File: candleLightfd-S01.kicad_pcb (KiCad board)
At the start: 2 copper layers, 37.7 x 20 mm, 45 parts, among them P1 CONN_01X02, P2 CONN_01X02, T101 Tab, T102 Tab, T103 Tab, T104 Tab, U1 STM32G0B1CBT, U2 MCP1754ST-3302E/MB, U3 TJA1051T3, U4 TJA1051T3, X1 629722000214_pasteInHole, X3 TC2030-NL, Y1 830055299

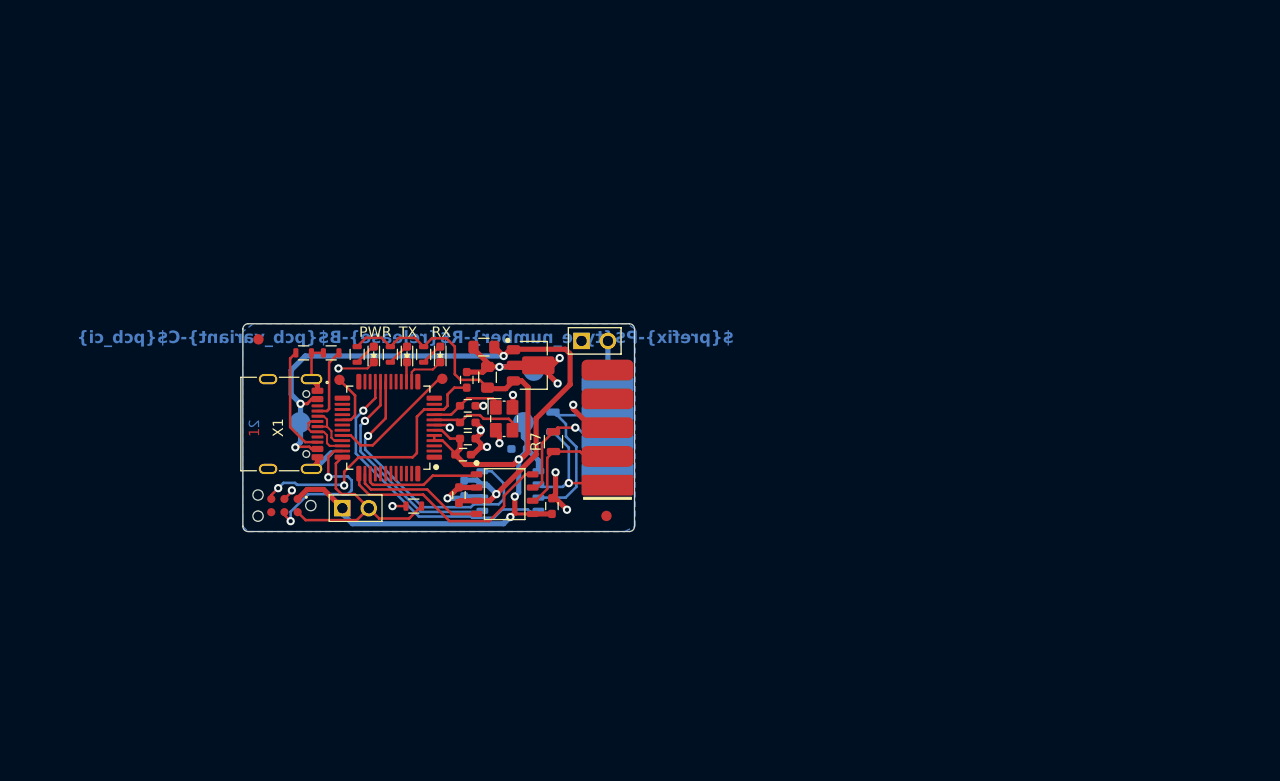
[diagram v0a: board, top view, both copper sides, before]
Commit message: clean up
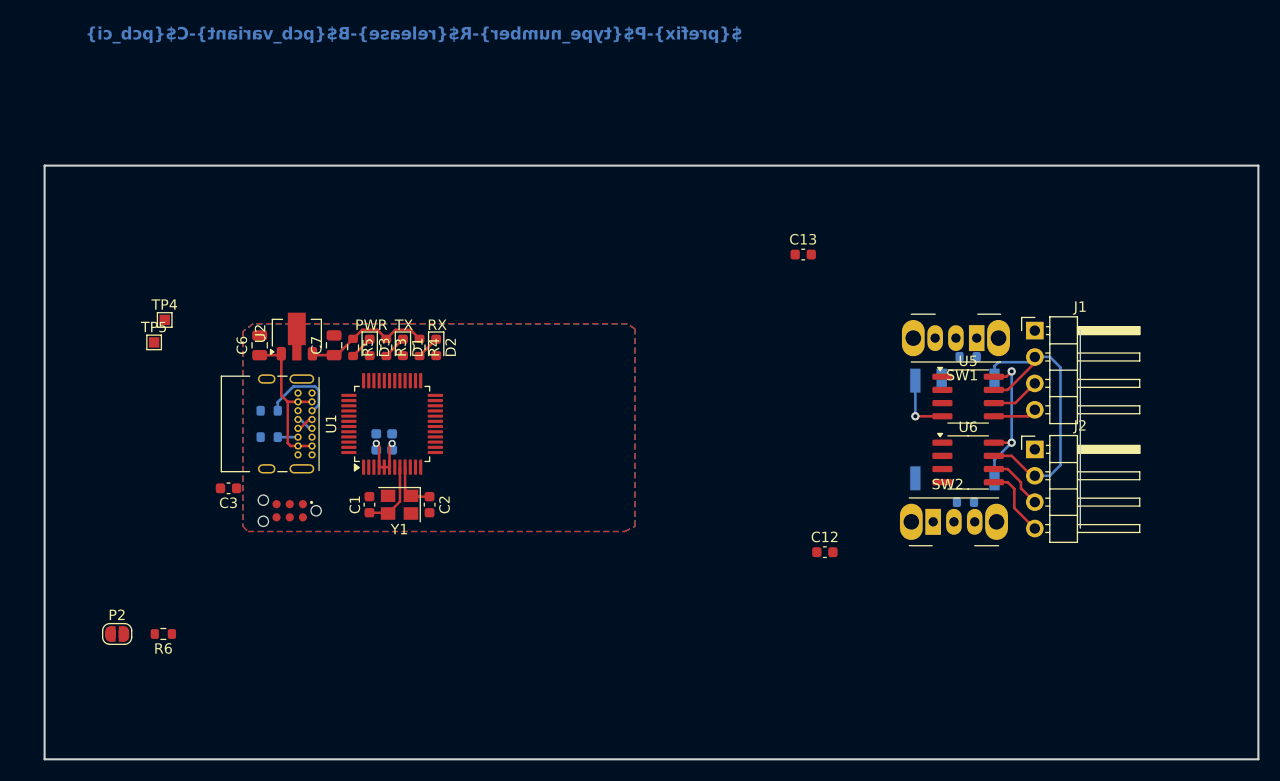
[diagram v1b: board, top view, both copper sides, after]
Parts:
- removed C10, C11, C8, C9: 100n_0603_X7R_10%_50V_-40C..125C_Chip-Capacitor, Capacitors_SMD:C_0603
- removed NB2: LAYERSTACK_TB, mechanical:LAYERSTACK_TB
- removed NB3, NB4: Passermarke_1mm_1.8mmx1.8mm, mechanical:Passermarke_1mm_1.8mmx1.8mm
- removed P1: CONN_01X02, Connector_generic:Header_1x2_Pitch2.54mm
- removed R1, R2: 5k1_0603_100mW_1%_E24_Chip-Resistor, Resistors_SMD:R_0603
- removed T101, T102, T103, T104: Tab, kikit:Tab
- removed TP1, TP2, TP3: TP2.0mm, Connector_generic:TP2.0mm
- removed U3, U4: TJA1051T3, tssop:SOIC-8_3.90mmx4.90mm_Pitch1.27mm
- removed X1: 629722000214_pasteInHole, Socket_GCT:USB4105_pasteInHole
- removed X2: ~, d-sub:D-SUB-9_side
- added C12: 100n_0603_X7R_10%_50V_-40C..125C_Chip-Capacitor, Capacitor_SMD:C_0603_1608Metric, F.Cu at (157.0, 142.0)
- added C13: 100n_0603_X7R_10%_50V_-40C..125C_Chip-Capacitor, Capacitor_SMD:C_0603_1608Metric, F.Cu at (154.9, 113.3)
- added J1: CAN1, Connector_PinHeader_2.54mm:PinHeader_1x04_P2.54mm_Horizontal, F.Cu at (177.2, 120.7)
- added J2: CAN2, Connector_PinHeader_2.54mm:PinHeader_1x04_P2.54mm_Horizontal, F.Cu at (177.2, 132.1)
- added J3: USB_C_Receptacle_USB2.0_16P, Connector_USB:USB_C_Receptacle_GCT_USB4085, F.Cu at (107.7, 126.7)
- added R10: 5k1_0603_100mW_1%_E24_Chip-Resistor, Resistor_SMD:R_0603_1608Metric, B.Cu at (103.5, 128.4)
- added R9: 5k1_0603_100mW_1%_E24_Chip-Resistor, Resistor_SMD:R_0603_1608Metric, B.Cu at (103.5, 130.9)
- added SW1: Term1, Button_Switch_THT:SW_Slide_SPDT_Angled_CK_OS102011MA1Q, F.Cu at (171.6, 121.4)
- added SW2: Term2, Button_Switch_THT:SW_Slide_SPDT_Angled_CK_OS102011MA1Q, F.Cu at (167.4, 139.1)
- added U5: ISO1044BD, Package_SO:SOIC-8_3.9x4.9mm_P1.27mm, F.Cu at (170.8, 127.0)
- added U6: ISO1044BD, Package_SO:SOIC-8_3.9x4.9mm_P1.27mm, F.Cu at (170.8, 133.3)
- added U7: NXE1S0505MC, Converter_DCDC:Converter_DCDC_Murata_NXExSxxxxMC_SMD, B.Cu at (170.8, 130.2)
- C1, C2, C3: footprint Capacitors_SMD:C_0603 -> Capacitor_SMD:C_0603_1608Metric
- C4, C5: footprint Capacitors_SMD:C_0603 -> Capacitor_SMD:C_0603_1608Metric; moved to B.Cu
- C6, C7: footprint Capacitors_SMD:C_0805 -> Capacitor_SMD:C_0805_2012Metric
- D1, D2, D3: footprint LEDs_Kingbright:LED_Kingbright_0603 -> LED_SMD:LED_0603_1608Metric
- P2: footprint Connector_generic:Header_1x2_Pitch2.54mm -> Jumper:SolderJumper-2_P1.3mm_Open_RoundedPad1.0x1.5mm
- R3, R4, R5, R6: footprint Resistors_SMD:R_0603 -> Resistor_SMD:R_0603_1608Metric
- R7: value 120R_0805_125mW_1%_E24_Chip-Resistor -> 120; footprint Resistors_SMD:R_0805 -> Resistor_SMD:R_0603_1608Metric; moved to B.Cu
- R8: value 120R_0805_125mW_1%_E24_Chip-Resistor -> 120; footprint Resistors_SMD:R_0805 -> Resistor_SMD:R_0603_1608Metric
- TP4, TP5: footprint Connector_generic:TP1.0mm -> TestPoint:TestPoint_Pad_1.0x1.0mm
- U1: footprint QFP:LQFP-48_7mmx7mm_Pitch0.5mm -> Package_QFP:LQFP-48_7x7mm_P0.5mm
- U2: footprint TO_SMD:SOT-89 -> Package_TO_SOT_SMD:SOT-89-3
- Y1: value 830055299 -> 830108313809; footprint crystal:Crystal_4Pin_SMD_3.2mmx2.5mm -> Crystal:Crystal_SMD_3225-4Pin_3.2x2.5mm
- moved NB1 79.4 mm to (45.1, 94.6)
- moved R7 40.7 mm to (170.8, 123.2), turned to 180 degrees
- moved R8 40.5 mm to (170.6, 137.2), turned to 180 degrees
- moved TP4 27.3 mm to (93.5, 119.6)
- moved P2 27.1 mm to (88.9, 149.9)
- moved R6 27.1 mm to (93.3, 149.9)
- moved C3 25.2 mm to (99.6, 135.8), turned to 180 degrees
- moved U2 23.0 mm to (106.2, 120.9), turned to 90 degrees
- moved C6 21.6 mm to (102.6, 122.1), turned to 90 degrees
- moved TP5 18.2 mm to (92.5, 121.8)
- moved C7 15.1 mm to (109.8, 122.1)
- moved Y1 13.0 mm to (116.1, 137.4), turned to 180 degrees
- moved C1 12.3 mm to (113.2, 137.4), turned to -90 degrees
- moved C2 10.2 mm to (119.0, 137.4), turned to 90 degrees
- moved C4 8.45 mm to (113.8, 131.4), turned to 90 degrees
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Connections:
- R7 pad 2: /CAN1_L -> Net-(SW1-B)
- R8 pad 2: /CAN2_L -> Net-(SW2-B)
- U1 pad 19: /CAN Transiver/CAN2_RX -> /CAN Transceiver/CAN2_RX
- U1 pad 20: /CAN Transiver/CAN2_TX -> /CAN Transceiver/CAN2_TX
- U1 pad 21: /CAN Transiver/CAN2_S -> unconnected-(U1B-PB2-Pad21)
- U1 pad 37: /CAN Transiver/CAN1_S -> unconnected-(U1A-PA15-Pad37)
- U1 pad 38: /CAN Transiver/CAN1_RX -> /CAN Transceiver/CAN1_RX
- U1 pad 39: /CAN Transiver/CAN1_TX -> /CAN Transceiver/CAN1_TX
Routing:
- net +3V3: track 83.2 -> 19.5 mm, vias 3 -> 2
- net +5V: track 65.2 -> 15.8 mm, vias 4 -> 0
- net GND: track 54.9 -> 6.09 mm, vias 16 -> 1
- net GNDD: track 0.00 -> 31.1 mm
- net /CAN Transiver/CAN2_S: track 28.3 -> 0.00 mm, vias 1 -> 0
- net /CAN Transiver/CAN2_RX: track 27.4 -> 0.00 mm, vias 1 -> 0
- net /MCU/NRST: track 27.2 -> 0.00 mm, vias 2 -> 0
- net /CAN Transiver/CAN1_S: track 21.7 -> 0.00 mm
- net /CAN Transiver/CAN2_TX: track 21.7 -> 0.00 mm, vias 1 -> 0
- net /MCU/SWCLK: track 20.9 -> 0.00 mm
- net /MCU/SWDIO: track 15.7 -> 0.00 mm, vias 2 -> 0
- net +5VD: track 0.00 -> 14.6 mm, vias 0 -> 2
- net /CAN Transiver/CAN1_RX: track 12.9 -> 0.00 mm
- net /MCU/RX: track 12.7 -> 0.00 mm
- net /CAN2_H: track 17.7 -> 5.60 mm
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- added copper zone on F.Cu, net GND
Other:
- board size 37.7 x 20 mm -> 116.8 x 57.2 mm
- board text removed: "+3V3"
- board text removed: "0"
- board text removed: "0 mm"
- board text removed: "0.01 mm"
- board text removed: "0.02"
- board text removed: "0.035 mm"
- board text removed: "1"
- board text removed: "1.51 mm"
- board text removed: "12V"
- board text removed: "3.3"
- board text removed: "4.5"
- board text removed: "5V"
- board text removed: "B.Cu"
- board text removed: "B.Mask"
- board text removed: "B.Paste"
- board text removed: "B.Silkscreen"
- board text removed: "Black"
- board text removed: "Bottom Silk Screen"
- board text removed: "Bottom Solder Mask"
- board text removed: "Bottom Solder Paste"
- board text removed: "Color"
- board text removed: "Dielectric 1"
- board text removed: "Epsilon R"
- board text removed: "F.Cu"
- board text removed: "F.Mask"
- board text removed: "F.Paste"
- board text removed: "F.Silkscreen"
- board text removed: "FR4"
- board text removed: "GND"
- board text removed: "Layer Name"
- board text removed: "Loss Tangent"
- board text removed: "Material"
- board text removed: "Not specified"
- board text removed: "Thickness (mm)"
- board text removed: "Top Silk Screen"
- board text removed: "Top Solder Mask"
- board text removed: "Top Solder Paste"
- board text removed: "Type"
- board text removed: "White"
- board text removed: "copper"
- board text removed: "core"

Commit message: gsi-v1
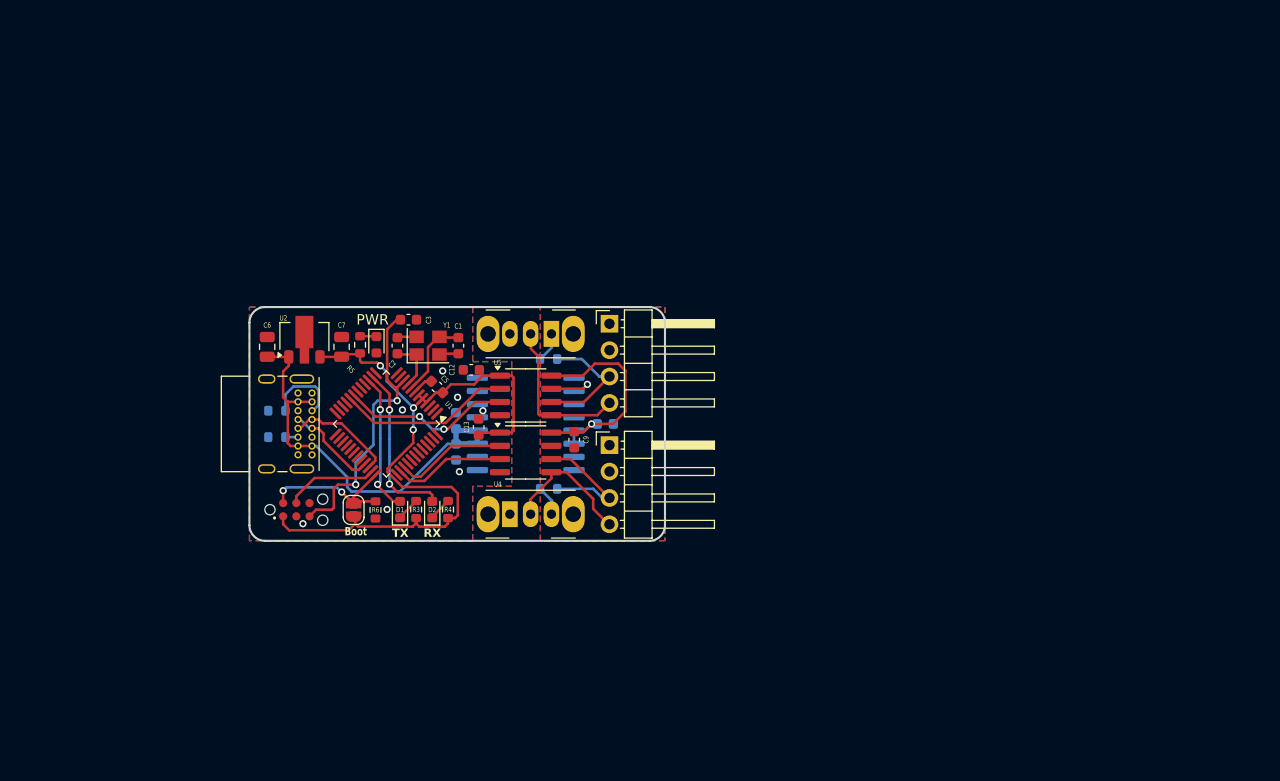
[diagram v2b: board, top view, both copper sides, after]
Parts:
- removed C4: 100n, Capacitor_SMD:C_0603_1608Metric
- removed TP4, TP5: TP1.0mm, TestPoint:TestPoint_Pad_1.0x1.0mm
- removed U6: ISO1044BD, Package_SO:SOIC-8_3.9x4.9mm_P1.27mm
- removed U7: NXE1S0505MC, Converter_DCDC:Converter_DCDC_Murata_NXExSxxxxMC_SMD
- added C10: 10u_0603_X7R_10%_50V_-40C..125C_Chip-Capacitor, Capacitor_SMD:C_0603_1608Metric, B.Cu at (121.5, 129.3)
- added C11: 100n_0603_X7R_10%_50V_-40C..125C_Chip-Capacitor, Capacitor_SMD:C_0603_1608Metric, B.Cu at (121.5, 132.3)
- added C8: 10u_0603_X7R_10%_50V_-40C..125C_Chip-Capacitor, Capacitor_SMD:C_0603_1608Metric, B.Cu at (135.9, 129.6)
- added C9: 100n_0603_X7R_10%_50V_-40C..125C_Chip-Capacitor, Capacitor_SMD:C_0603_1608Metric, F.Cu at (132.9, 131.2)
- added U3: R05CTE05S, Package_SO:SOIC-16W_7.5x10.3mm_P1.27mm, B.Cu at (128.2, 129.6)
- added U4: ISO1044BD, Package_SO:SOIC-8_3.9x4.9mm_P1.27mm, F.Cu at (128.2, 132.4)
- C5: moved to F.Cu
- C7: value 10u_0805_X7R_10%_10V_-40C..125C_Chip-Capacitor -> 1u_0805_X7R_10%_10V_-40C..125C_Chip-Capacitor
- moved NB1 78.4 mm to (115.1, 129.8), turned to 0 degrees
- moved SW1 48.0 mm to (126.7, 138.3), turned to 0 degrees
- moved J2 42.7 mm to (136.3, 120.0)
- moved U5 42.6 mm to (128.2, 126.9)
- moved R8 42.4 mm to (130.4, 123.4)
- moved J1 42.4 mm to (136.3, 131.7)
- moved R7 42.3 mm to (130.4, 135.9)
- moved SW2 41.0 mm to (130.7, 121.0), turned to 180 degrees
- moved C12 38.3 mm to (123.0, 124.4), turned to 180 degrees
- moved C13 35.4 mm to (123.7, 129.9), turned to 90 degrees
- moved P2 25.7 mm to (111.7, 137.9), turned to 90 degrees
- moved C3 23.7 mm to (116.9, 119.6), turned to 0 degrees
- moved R6 23.7 mm to (113.8, 137.9), turned to -90 degrees
- moved C1 17.5 mm to (121.7, 122.1), turned to 90 degrees
- moved R3 15.9 mm to (117.7, 137.9), turned to 90 degrees
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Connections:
- R7 pad 2: Net-(SW1-B) -> Net-(SW1-C)
- R8 pad 2: Net-(SW2-B) -> Net-(SW2-A)
- SW1 pad 1: /CAN1_L -> unconnected-(SW1-A-Pad1)
- SW1 pad 2: Net-(SW1-B) -> /CAN1_L
- SW1 pad 3: unconnected-(SW1-C-Pad3) -> Net-(SW1-C)
- SW2 pad 1: /CAN2_L -> Net-(SW2-A)
- SW2 pad 2: Net-(SW2-B) -> /CAN2_L
- U1 pad 29: /MCU/TX -> unconnected-(U1A-PA9-Pad29)
- U1 pad 32: /MCU/RX -> unconnected-(U1A-PA10-Pad32)
- U5 pad 2: /CAN Transceiver/CAN1_TX -> /CAN Transceiver/CAN2_TX
- U5 pad 3: /CAN Transceiver/CAN1_RX -> /CAN Transceiver/CAN2_RX
- U5 pad 5: /CAN1_L -> /CAN2_L
- U5 pad 6: /CAN1_H -> /CAN2_H
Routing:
- net +3V3: track 19.5 -> 71.3 mm, vias 2 -> 3
- net GNDD: track 31.1 -> 3.64 mm, vias 0 -> 1
- net /MCU/NRST: track 0.00 -> 27.4 mm, vias 0 -> 2
- net +5V: track 15.8 -> 40.6 mm
- net /CAN Transceiver/CAN2_TX: track 0.00 -> 16.7 mm
- net /MCU/LED_RX: track 0.00 -> 16.6 mm, vias 0 -> 2
- net /CAN Transceiver/CAN2_RX: track 0.00 -> 16.5 mm, vias 0 -> 2
- net /MCU/SWCLK: track 0.00 -> 14.6 mm, vias 0 -> 2
- net /MCU/LED_TX: track 0.07 -> 13.5 mm, vias 0 -> 2
- net /CAN Transceiver/CAN1_RX: track 0.00 -> 10.9 mm
- net /CAN Transceiver/CAN1_TX: track 0.00 -> 10.8 mm
- net /CAN1_L: track 4.20 -> 13.7 mm
- net /MCU/SWDIO: track 0.00 -> 8.97 mm
- net +5VD: track 14.6 -> 23.5 mm, vias 2 -> 1
- net /USB_P: track 1.70 -> 10.5 mm
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- added copper zone on B.Cu, net GNDD
- added copper zone on F.Cu, net GNDD
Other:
- board size 116.8 x 57.2 mm -> 40 x 22.5 mm
- board text added: "CAN 1"
- board text added: "CAN 2"
- board text added: "GSI GmbH v 1.0 10/2024"
- board text added: "candlelightFD"
- board text added: "x G H L"
- board text removed: "${prefix}-P${type_number}-R${release}-B${pcb_variant}-C${pcb_ci}"
